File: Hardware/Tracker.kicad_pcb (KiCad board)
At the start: 2 copper layers, 63.8 x 80.7 mm, 43 parts, among them J1 Battery, J10 132134, J11 SPI_Programming, J12 Battery, J3 Wind, J4 RX, J5 TX, J6 GND, J7 GND, J8 GND, J9 Header_LED, U1 L7805, U2 ATmega328P-P, U3 LM317_TO-220, U7 GK9501, U9 L298N, Y1 16MHz

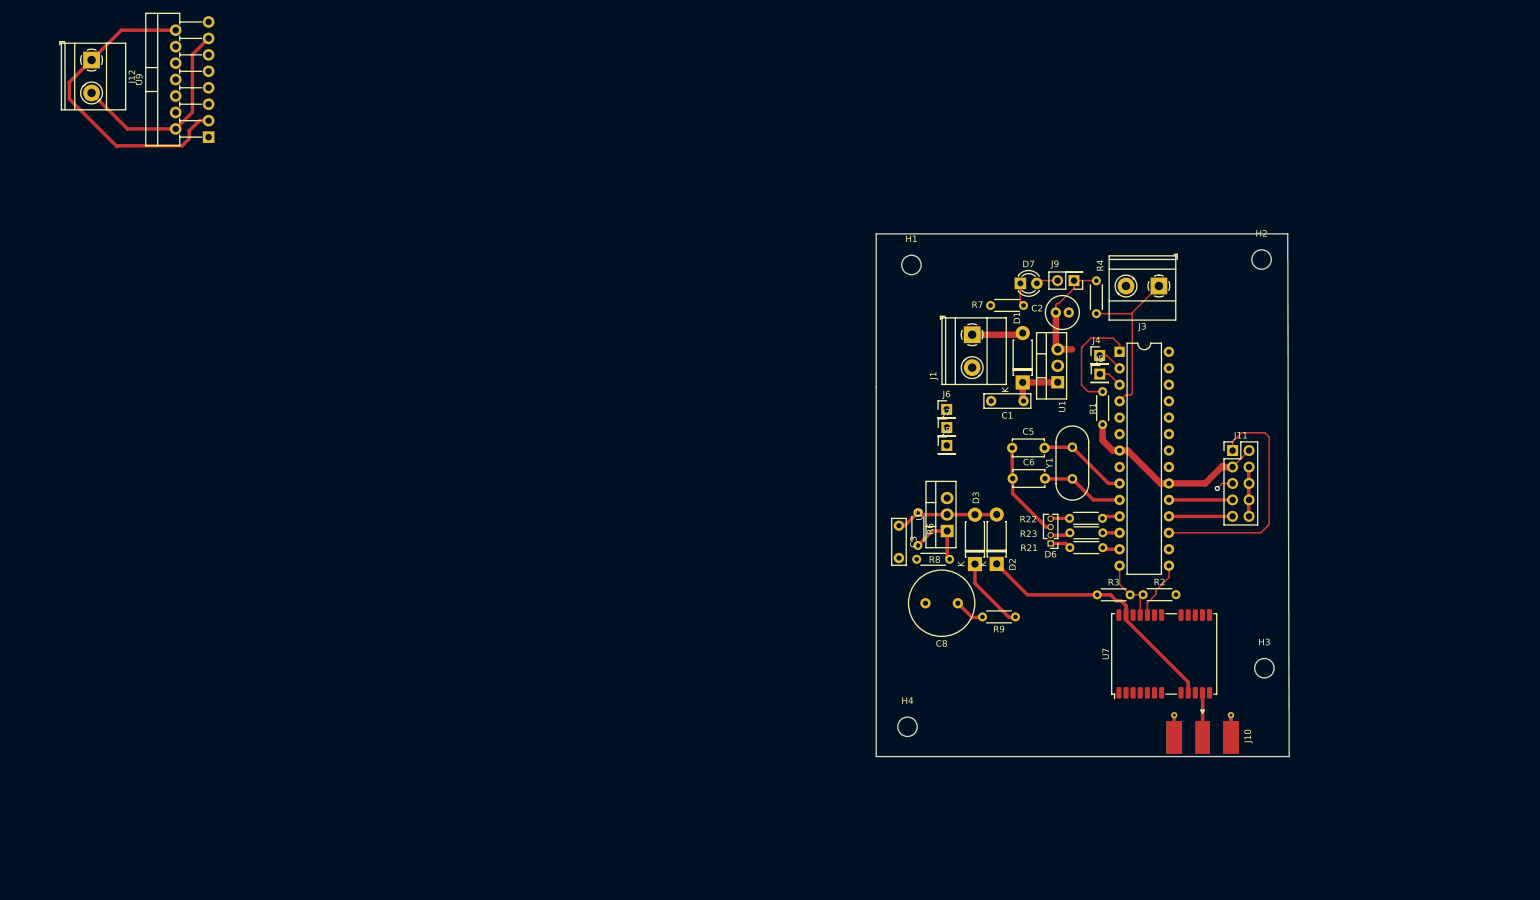
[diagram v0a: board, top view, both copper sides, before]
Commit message: update of directory
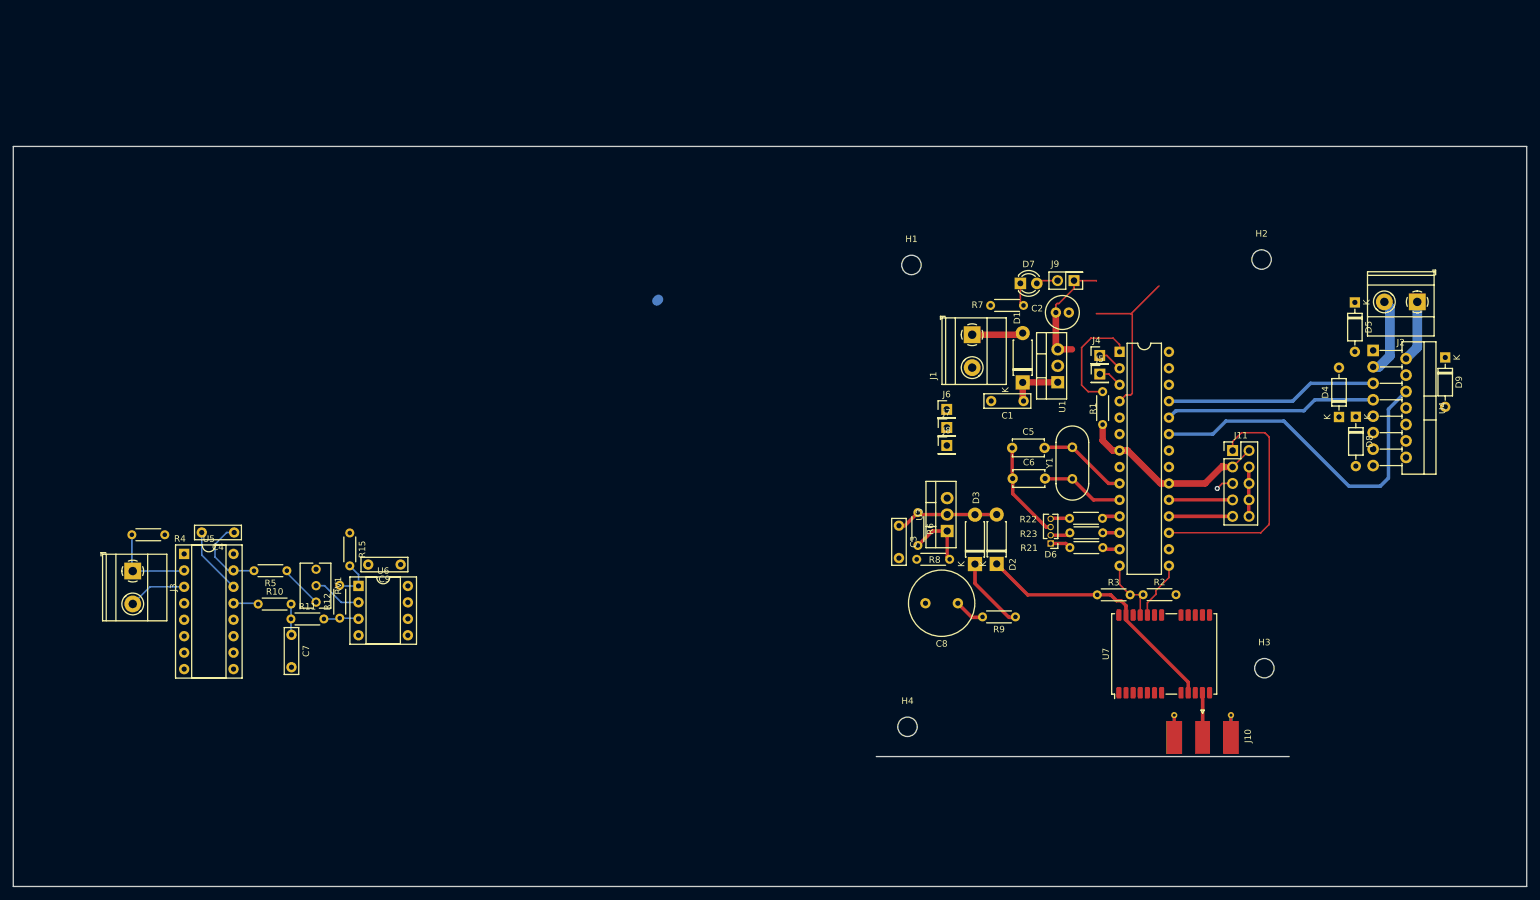
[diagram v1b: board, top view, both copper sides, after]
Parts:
- removed J12: Battery, TerminalBlock_Phoenix:TerminalBlock_Phoenix_MKDS-1,5-2-5.08_1x02_P5.08mm_Horizontal
- removed U9: L298N, Package_TO_SOT_THT:TO-220-15_P2.54x2.54mm_StaggerOdd_Lead4.58mm_Vertical
- added C4: 100nF, Capacitor_THT:C_Rect_L7.0mm_W2.0mm_P5.00mm, F.Cu at (39.2, 98.3)
- added C7: 100nF, Capacitor_THT:C_Rect_L7.0mm_W2.0mm_P5.00mm, F.Cu at (48.0, 114.2)
- added C9: 100nF, Capacitor_THT:C_Rect_L7.0mm_W2.0mm_P5.00mm, F.Cu at (64.9, 103.3)
- added D4: 1N4148, Diode_THT:D_DO-35_SOD27_P7.62mm_Horizontal, F.Cu at (209.8, 80.5)
- added D5: 1N4148, Diode_THT:D_DO-35_SOD27_P7.62mm_Horizontal, F.Cu at (212.2, 62.8)
- added D8: 1N4148, Diode_THT:D_DO-35_SOD27_P7.62mm_Horizontal, F.Cu at (212.4, 80.5)
- added D9: 1N4148, Diode_THT:D_DO-35_SOD27_P7.62mm_Horizontal, F.Cu at (226.2, 71.3)
- added J2: Motor, TerminalBlock_Phoenix:TerminalBlock_Phoenix_MKDS-1,5-2-5.08_1x02_P5.08mm_Horizontal, F.Cu at (221.8, 62.8)
- added R10: 10k, Resistor_THT:R_Axial_DIN0204_L3.6mm_D1.6mm_P5.08mm_Horizontal, F.Cu at (42.9, 109.4)
- added R11: 10k, Resistor_THT:R_Axial_DIN0204_L3.6mm_D1.6mm_P5.08mm_Horizontal, F.Cu at (48.0, 111.7)
- added R12: 10k, Resistor_THT:R_Axial_DIN0204_L3.6mm_D1.6mm_P5.08mm_Horizontal, F.Cu at (55.5, 111.6)
- added R15: 10k, Resistor_THT:R_Axial_DIN0204_L3.6mm_D1.6mm_P5.08mm_Horizontal, F.Cu at (57.0, 98.4)
- added R5: 10k, Resistor_THT:R_Axial_DIN0204_L3.6mm_D1.6mm_P5.08mm_Horizontal, F.Cu at (47.3, 104.2)
- added RV1: R_Potentiometer, Potentiometer_THT:Potentiometer_Bourns_3266Y_Vertical, F.Cu at (51.9, 109.1)
- added U4: L298N, Package_TO_SOT_THT:TO-220-15_P2.54x2.54mm_StaggerOdd_Lead4.58mm_Vertical, F.Cu at (215.0, 70.2)
- added U5: 74HC123, Package_DIP:DIP-16_W7.62mm_Socket, F.Cu at (31.5, 101.7)
- added U6: LM358, Package_DIP:DIP-8_W7.62mm_Socket, F.Cu at (58.4, 106.6)
- J9: value Header_LED -> Haeder_LED
- moved J3 164.4 mm to (23.5, 104.3), turned to -90 degrees
- moved R4 149.1 mm to (28.5, 98.7), turned to 180 degrees
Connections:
- net /WIND/OUT renamed /WIND/RAW_DATA
- U2 pad 23: unconnected-(U2-PC0-Pad23) -> /Motors/EN_MOTOR
- U2 pad 24: unconnected-(U2-PC1-Pad24) -> /Motors/IN2_MOTOR
- U2 pad 25: unconnected-(U2-PC2-Pad25) -> /Motors/IN1_MOTOR
- U2 pad 5: unconnected-(U2-PD3-Pad5) -> /WIND/Wind_interrupt
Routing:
- net /Motors/EN_MOTOR: track 0.00 -> 53.9 mm
- net Net-(J12-Pin_1): track 49.2 -> 0.00 mm
- net /Motors/IN1_MOTOR: track 0.00 -> 32.7 mm
- net /Motors/IN2_MOTOR: track 0.00 -> 32.7 mm
- net Net-(J12-Pin_2): track 31.4 -> 0.00 mm
- net /WIND/RAW_DATA: track 26.3 -> 39.9 mm
- net Net-(U5A-RCext): track 0.00 -> 12.6 mm
- net Net-(D4-A): track 0.00 -> 12.3 mm
- net Net-(U5A-Cext): track 0.00 -> 10.4 mm
- net Net-(D8-A): track 0.00 -> 9.48 mm
- net GND: track 22.7 -> 31.7 mm
- net Net-(U6A--): track 0.00 -> 7.62 mm
- net +5V: track 47.8 -> 54.5 mm
- net /WIND/Wind_interrupt: track 0.00 -> 6.60 mm
- net Net-(U6A-+): track 0.00 -> 5.44 mm
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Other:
- board size 63.8 x 80.7 mm -> 233.7 x 114.2 mm
